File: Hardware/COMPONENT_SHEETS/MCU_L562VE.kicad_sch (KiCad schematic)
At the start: 29 parts, among them SW1 MCU Reset, U7 STM32L562VET6Q, Y3 32MHz

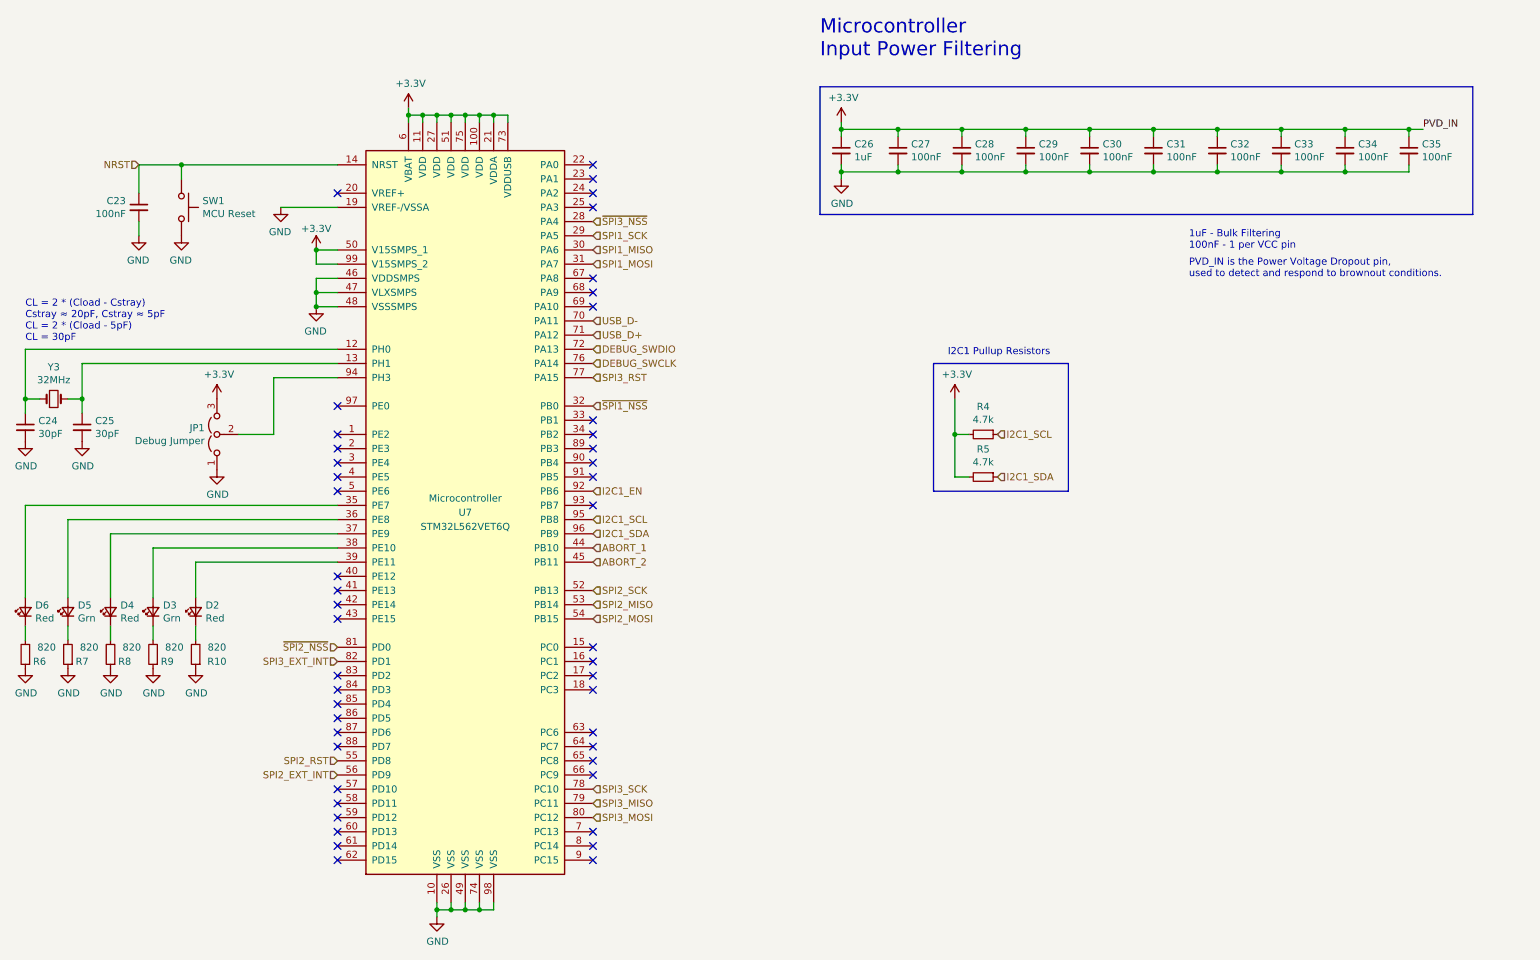
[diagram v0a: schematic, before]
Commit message: Corrected microcontroller component sheet
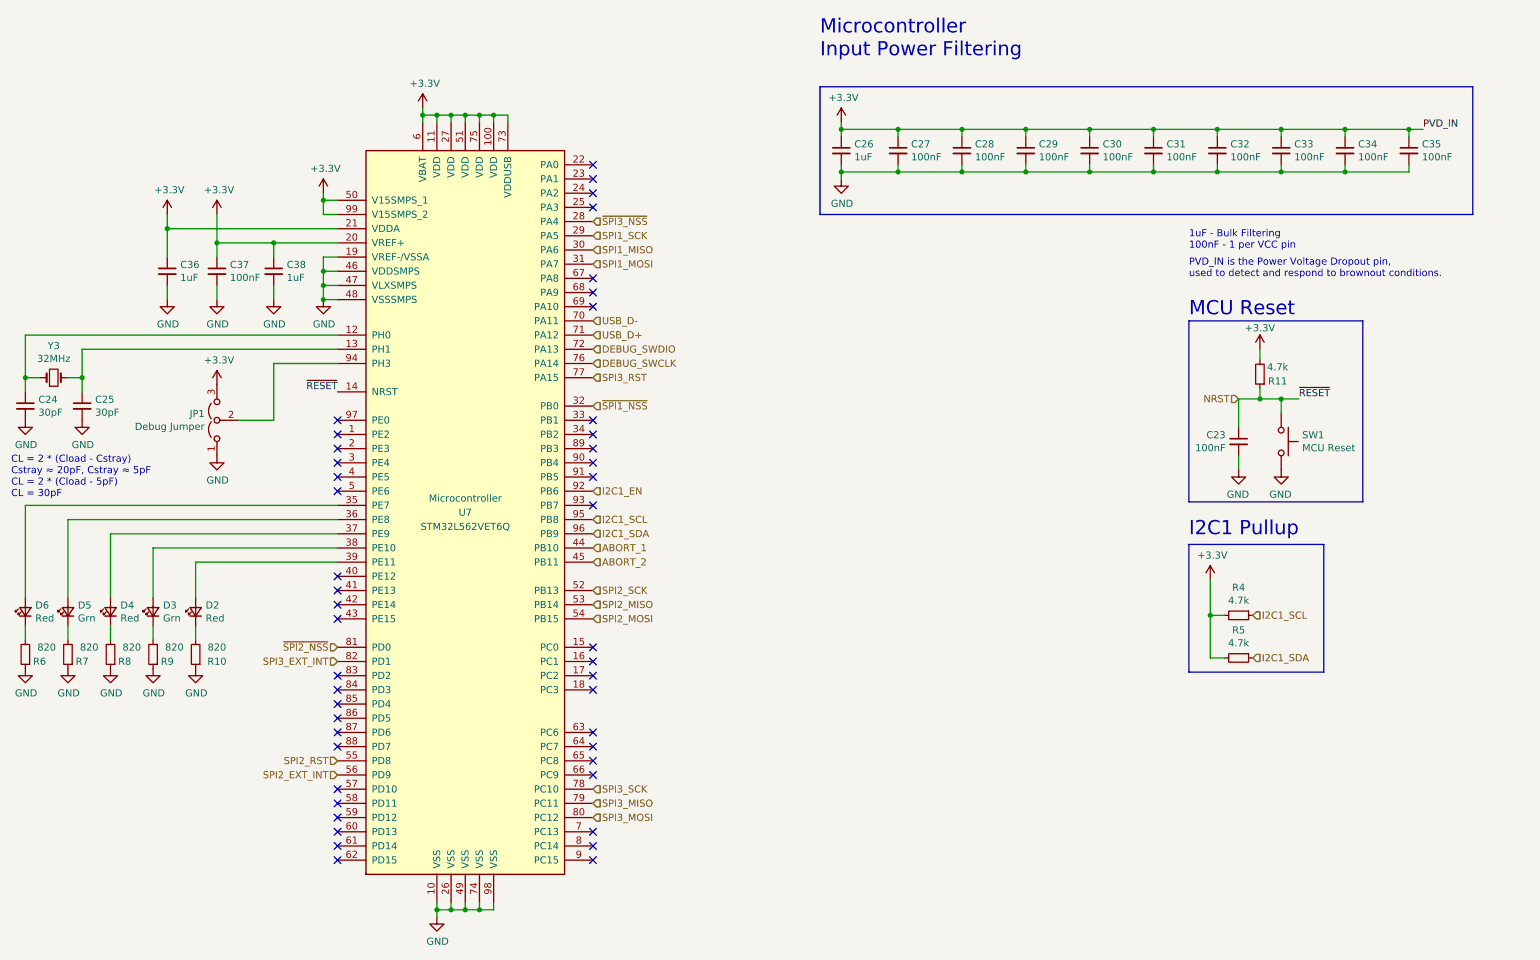
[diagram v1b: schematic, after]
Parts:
- added C36, C38: 1uF, Capacitor_SMD:C_0603_1608Metric_Pad1.08x0.95mm_HandSolder, symbol Device:C_Small
- added C37: 100nF, Capacitor_SMD:C_0603_1608Metric_Pad1.08x0.95mm_HandSolder, symbol Device:C_Small
- added R11: 4.7k, Resistor_SMD:R_0603_1608Metric_Pad1.05x0.95mm_HandSolder, symbol Device:R_Small
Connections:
- net +3V3: now also U7.20 (VREF+), C36.1, C37.1, C38.1, R11.2
- net GND: now also C36.2, C37.2, C38.2
- net NRST: now also R11.1
- no-connect marks 47 -> 46
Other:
- note added: "I2C1 Pullup"
- note added: "MCU Reset"
- note removed: "I2C1 Pullup Resistors"
- moved on the sheet: C23, C24, C25, JP1, R4, R5, SW1, Y3
